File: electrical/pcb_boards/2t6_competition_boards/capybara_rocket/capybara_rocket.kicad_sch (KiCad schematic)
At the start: 110 parts, among them J1 3.6V Battery, J10 Elevator, J11 SparkFun MAX-M10S, J12 Aileron 1, J13 Aileron 2, J14 Ground Camera, J15 Payload Camera, J16 DC Motor, J2 1.2V Battery, J3 3.6V Switch, J4 1.2V Switch, J5 LED, J6 NC, J7 CC, J8 VL53L1-SATEL, J9 Egg, Q1 SI4435DDY, Q2 SI4435DDY, U1 DS1307+, U10 TPS3839, U11 MP3414, U12 SN74LVC1G04, U13 MCP1640, U14 TPS3839, U15 STM32 NUCLEO-G431KB, U16 SN74AUP1G04, U17 SparkFun XBee Explorer, U2 Adafruit BNO085, U3 TLC555, U4 EEPROM, U5 LTC3536, U6 LTC3536, U7 Adafruit BMP581, U8 DRV8212, U9 INA219, Y1 AB38T-32.768KHZ

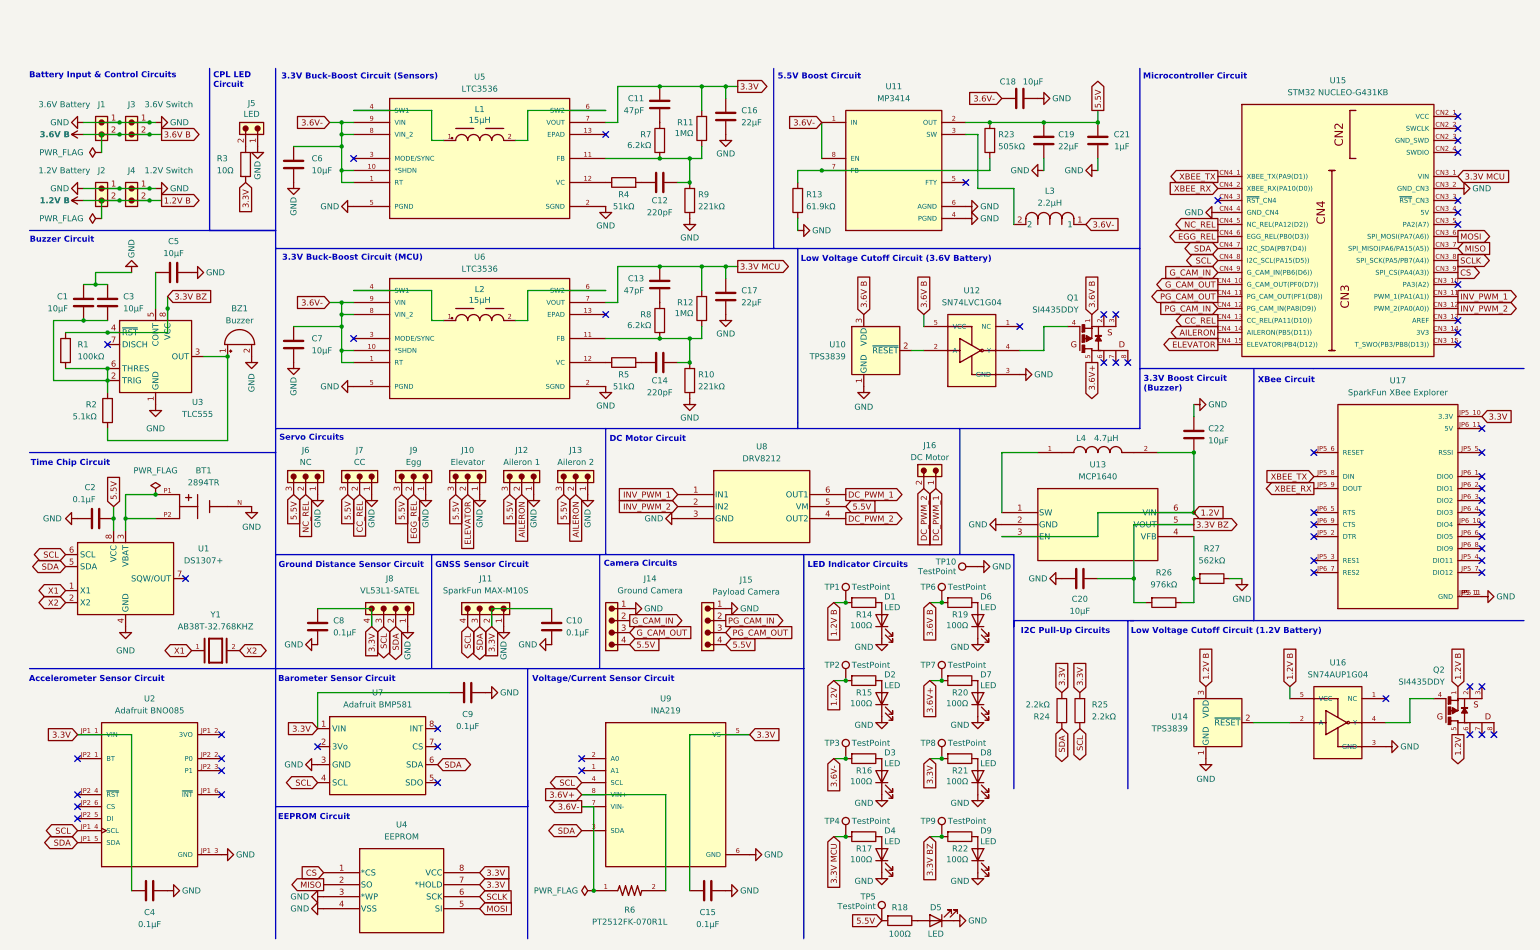
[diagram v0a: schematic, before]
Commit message: cpl pcb schematic review complete
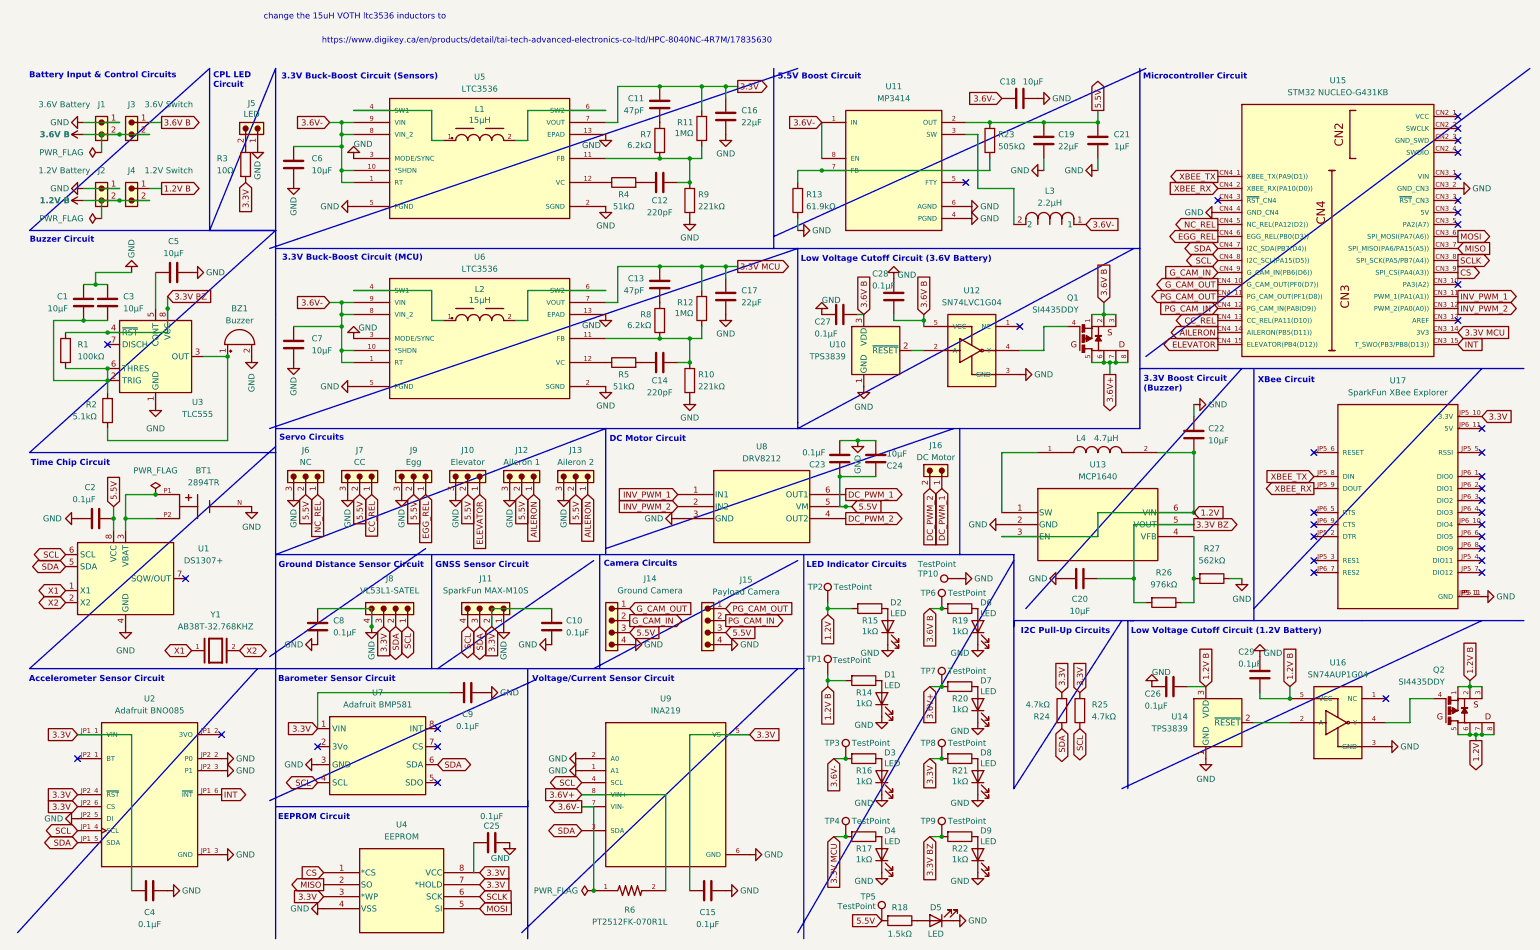
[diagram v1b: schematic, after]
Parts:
- added C23, C25, C26, C27, C28, C29: 0.1μF, Capacitor_SMD:C_0805_2012Metric_Pad1.18x1.45mm_HandSolder, symbol Device:C
- added C24: 10μF, Capacitor_SMD:C_1206_3216Metric_Pad1.33x1.80mm_HandSolder, symbol Device:C
- R14, R15, R16, R17, R19, R20, R21, R22: value 100Ω -> 1kΩ
- R18: value 100Ω -> 1.5kΩ
- R24, R25: value 2.2kΩ -> 4.7kΩ
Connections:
- net 1.2V: now also Q2.6, Q2.7, Q2.8
- net 1.2V B: now also J4.1, Q2.2, Q2.3, C26.1, C29.1
- net 3.3V: now also J8.3, U2.JP2_4 (~{RST}), U2.JP2_6 (CS), U4.3 (*WP); no longer C8.1, J8.4
- net 3.3V MCU: now also U15.CN3_14 (3V3); no longer U15.CN3_1 (VIN)
- net 3.6V B: now also J3.1, Q1.2, Q1.3, C27.1, C28.1
- net 3.6V+: now also Q1.6, Q1.7, Q1.8
- net 5.5V: now also J10.2, J12.2, J13.2, J14.3, J15.3, J6.2, J7.2, J9.2, C23.1, C24.1; no longer J10.3, J12.3, J13.3, J14.4, J15.4, J6.3, J7.3, J9.3
- net AILERON: now also J12.1, J13.1; no longer J12.2, J13.2
- net CC_REL: now also J7.1; no longer J7.2
- net EGG_REL: now also J9.1; no longer J9.2
- net ELEVATOR: now also J10.1; no longer J10.2
- net GND: now also C8.1, J10.3, J12.3, J13.3, J14.4, J15.4, J6.3, J7.3, J8.4, J9.3, U2.JP2_2 (P0), U2.JP2_3 (P1), U2.JP2_5 (DI), U5.13 (EPAD), U5.3 (MODE/SYNC), U6.13 (EPAD), U6.3 (MODE/SYNC), U9.1 (A1), U9.2 (A0), C23.2, C24.2, C25.2, C26.2, C27.2, C28.2, C29.2; no longer J10.1, J12.1, J13.1, J14.1, J15.1, J3.1, J4.1, J6.1, J7.1, J8.1, J9.1, U4.3 (*WP)
- net G_CAM_OUT: now also J14.1; no longer J14.3
- net NC_REL: now also J6.1; no longer J6.2
- net PG_CAM_OUT: now also J15.1; no longer J15.3
- net SCL: now also J8.1; no longer J8.3
- net INT: now reaches U2.JP1_6 (~{INT})
- net INT: now also U15.CN3_15 (T_SWO(PB3/PB8(D13)))
- no-connect marks 62 -> 39
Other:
- note added: "change the 15uH VOTH ltc3536 inductors to"
- note added: "https://www.digikey.ca/en/products/detail/tai-tech-advanced-electronics-co-ltd/HPC-8040NC-4R7M/17835630"
- moved on the sheet: D6, D7, J16, R19, R20, TP1, TP10, TP2, TP6, TP7
